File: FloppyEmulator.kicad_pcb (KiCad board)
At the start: 2 copper layers, 67.3 x 48.3 mm, 52 parts, among them Q1 Crystal_GND24, Q2 BC817, Q3 BC817, SW1 ALPS_5WAY, U1 STM32F405RGTx, U10 AP1117-15, U2 SN74LVC2G07, U3 SN74LVC2G07, U4 SN74LVC2G07, U5 SN74LVC2G07, U6 SN74LVC2G07, U7 SN74LVC2G07, U8 SN74LVC2G07, U9 SN74LVC2G07, X1 Micro_SD_Card_Det, X2 Conn_01x09, X3 Conn_02x17_Odd_Even, X4 TE 171826-4, X5 SWD

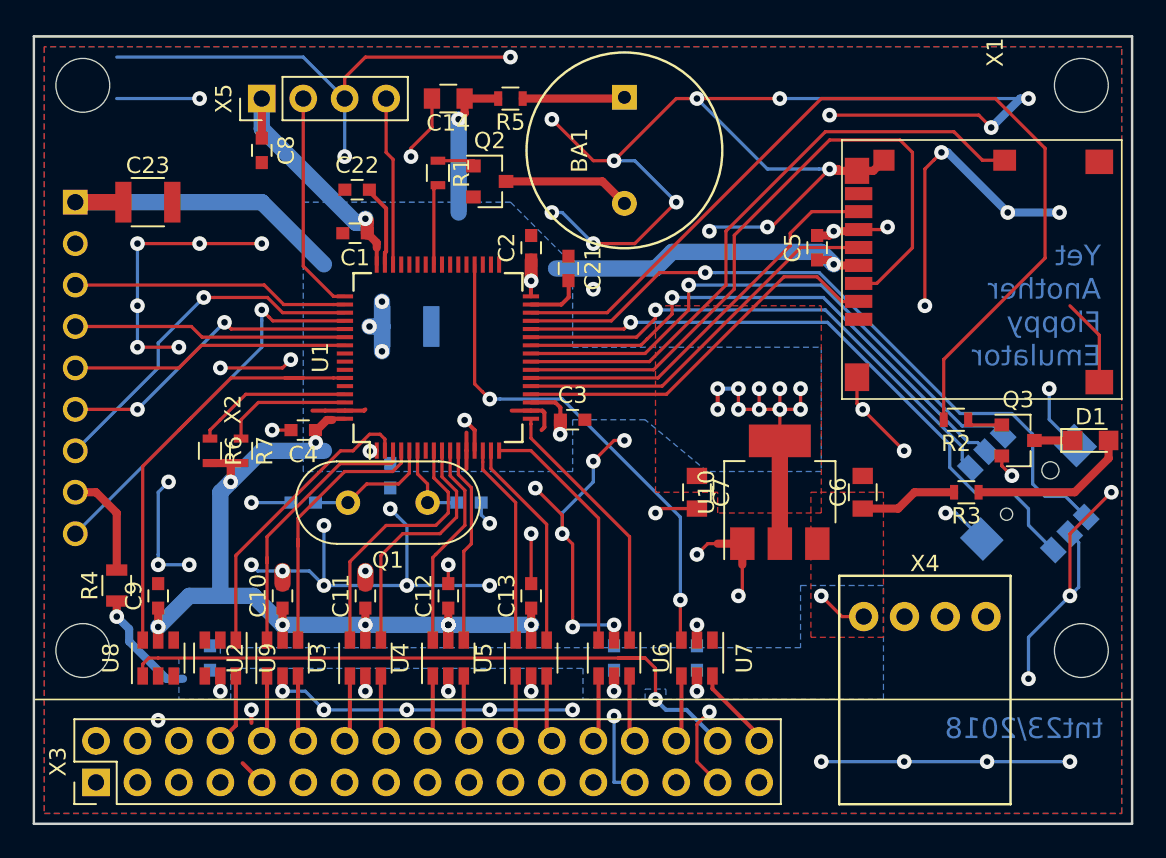
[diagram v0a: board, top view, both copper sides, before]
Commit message: More cleanups
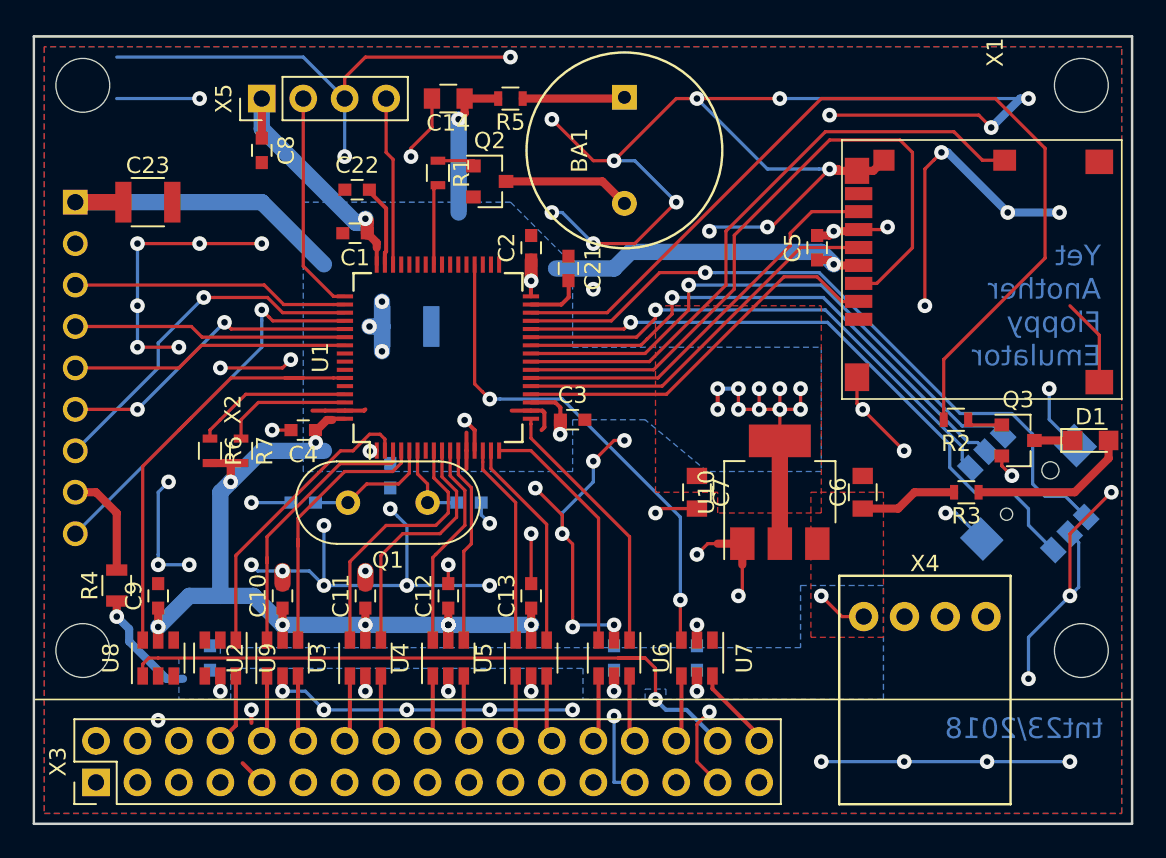
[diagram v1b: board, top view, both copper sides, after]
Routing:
- net (no net): track 1.09 -> 0.00 mm
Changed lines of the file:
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@@
     (thickness 1.6)
     (drawings 10)
-    (tracks 662)
+    (tracks 660)
     (zones 0)
     (modules 52)
@@
   (segment (start 172.72 96.35) (end 172.72 97.282) (width 0.5) (layer F.Cu) (net 8))
   (via (at 172.72 97.282) (size 0.9) (drill 0.4) (layers F.Cu B.Cu) (net 8))
+  (segment (start 177.8 71.374) (end 178.816 70.358) (width 1) (layer B.Cu) (net 9))
+  (segment (start 174.244 71.374) (end 177.8 71.374) (width 1) (layer B.Cu) (net 9))
+  (segment (start 190.5 70.358) (end 191.262 71.12) (width 1) (layer B.Cu) (net 9))
+  (segment (start 178.816 70.358) (end 190.5 70.358) (width 1) (layer B.Cu) (net 9))
   (segment (start 149.86 94.15) (end 149.86 93.345) (width 0.5) (layer F.Cu) (net 9))
   (segment (start 147.725 67.31) (end 144.78 67.31) (width 1) (layer F.Cu) (net 9))
@@
   (segment (start 163.255 82.535) (end 162.873662 82.535) (width 0.25) (layer F.Cu) (net 9))
   (via (at 162.836331 82.572331) (size 0.9) (drill 0.4) (layers F.Cu B.Cu) (net 9))
-  (segment (start 180.34 71.374) (end 181.356 70.358) (width 1) (layer B.Cu) (net 9))
-  (segment (start 190.5 70.358) (end 191.262 71.12) (width 1) (layer B.Cu) (net 9))
-  (segment (start 174.244 71.374) (end 180.34 71.374) (width 1) (layer B.Cu) (net 9))
-  (segment (start 181.356 70.358) (end 190.5 70.358) (width 1) (layer B.Cu) (net 9))
   (segment (start 168.275 62.23) (end 168.275 67.945) (width 1) (layer B.Cu) (net 9))
   (segment (start 168.64 61.865) (end 168.275 62.23) (width 0.5) (layer F.Cu) (net 9))
@@
   (segment (start 165.255 82.535) (end 165.255 83.919) (width 0.2) (layer F.Cu) (net 66))
   (via (at 180.34 97.790008) (size 0.9) (drill 0.4) (layers F.Cu B.Cu) (net 69))
-  (segment (start 146.37 95.57) (end 146.69 95.25) (width 0.25) (layer F.Cu) (net 0))
   (segment (start 153.35 100.01) (end 153.67 100.33) (width 0.25) (layer F.Cu) (net 70))
   (segment (start 181.356 74.168) (end 181.356 73.152) (width 0.2) (layer F.Cu) (net 75))
@@
   (segment (start 172.705 74.085) (end 177.375 74.085) (width 0.2) (layer F.Cu) (net 83))
   (segment (start 177.375 74.085) (end 190.5 60.96) (width 0.2) (layer F.Cu) (net 83))
-  (segment (start 145.415 93.345) (end 145.415 93.98) (width 0.5) (layer B.Cu) (net 0))
   (segment (start 150.368 96.52) (end 151.384 96.52) (width 0.5) (layer B.Cu) (net 84))
   (segment (start 148.082 94.234) (end 150.368 96.52) (width 0.5) (layer B.Cu) (net 84))
